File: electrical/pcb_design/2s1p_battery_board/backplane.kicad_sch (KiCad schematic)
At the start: 21 parts, among them J10 TE_Connectivity_7-5530843-7, J11 TE_Connectivity_7-5530843-7, J12 TE_Connectivity_7-5530843-7, J13 TE_Connectivity_7-5530843-7, J14 TE_Connectivity_7-5530843-7, J15 TE_Connectivity_7-5530843-7, J16 TE_Connectivity_7-5530843-7, J9 TE_Connectivity_7-5530843-7, U3 TCAN330

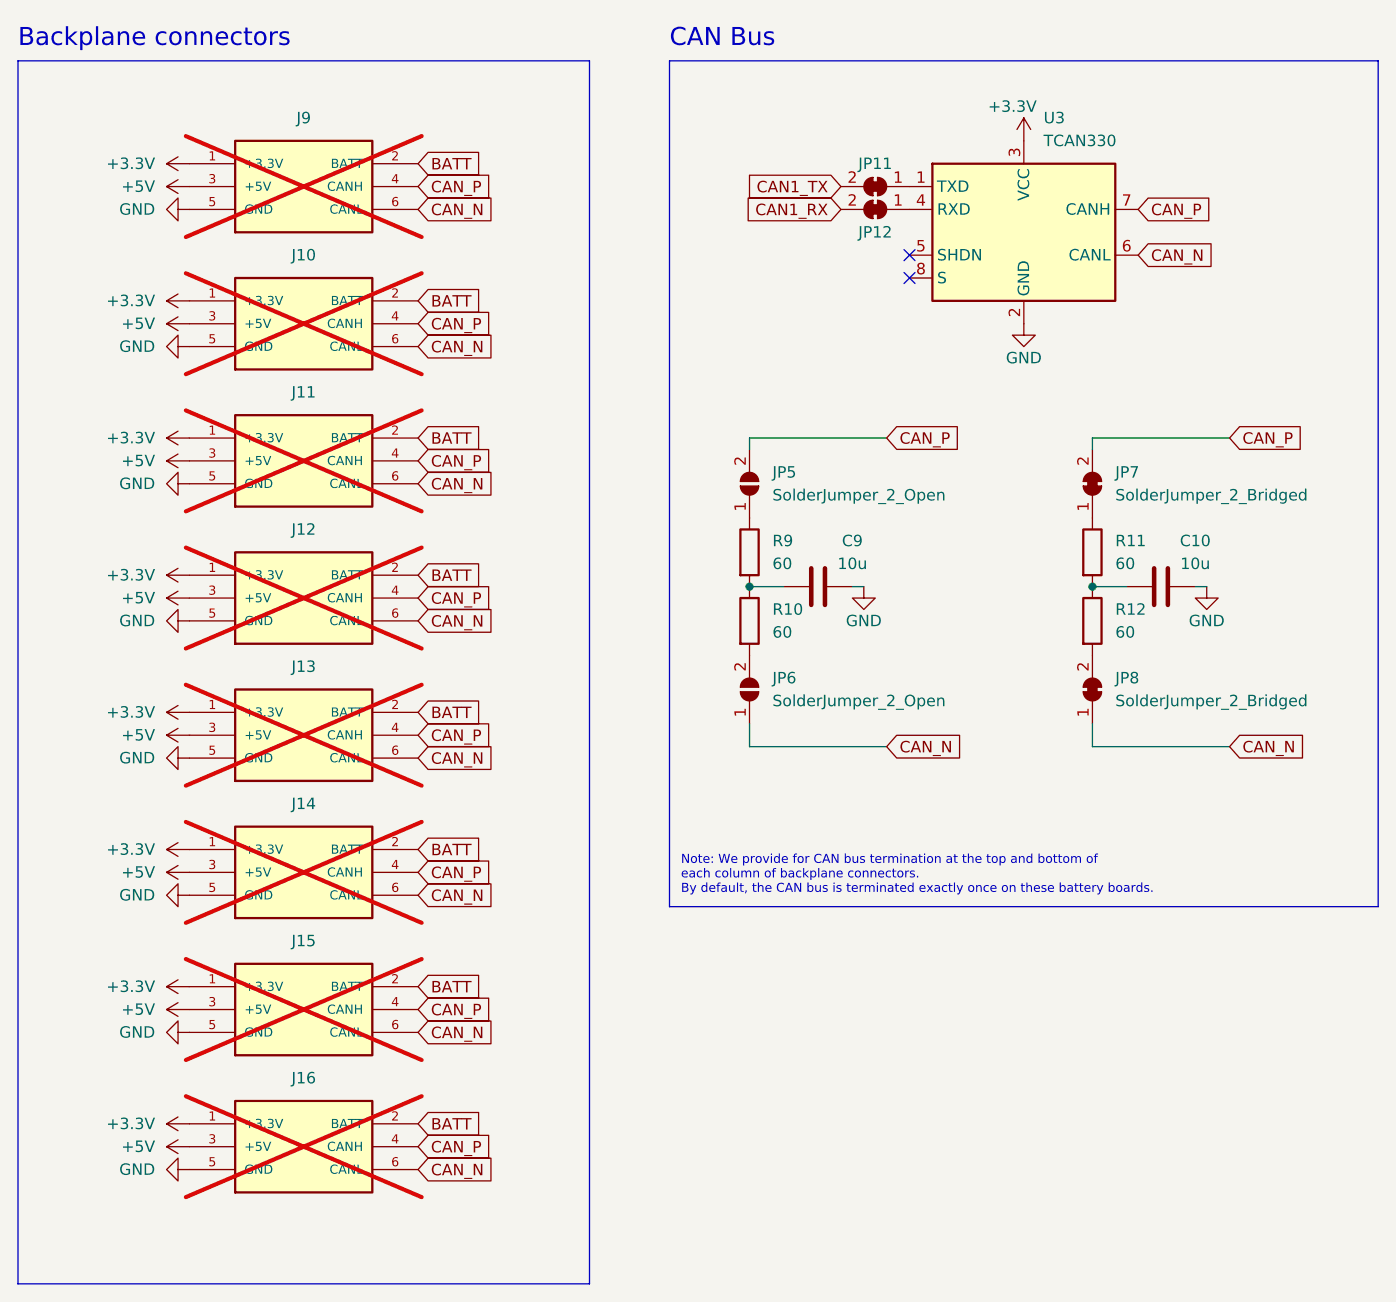
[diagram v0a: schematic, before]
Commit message: Checkpointing work rearranging backplane pin-out
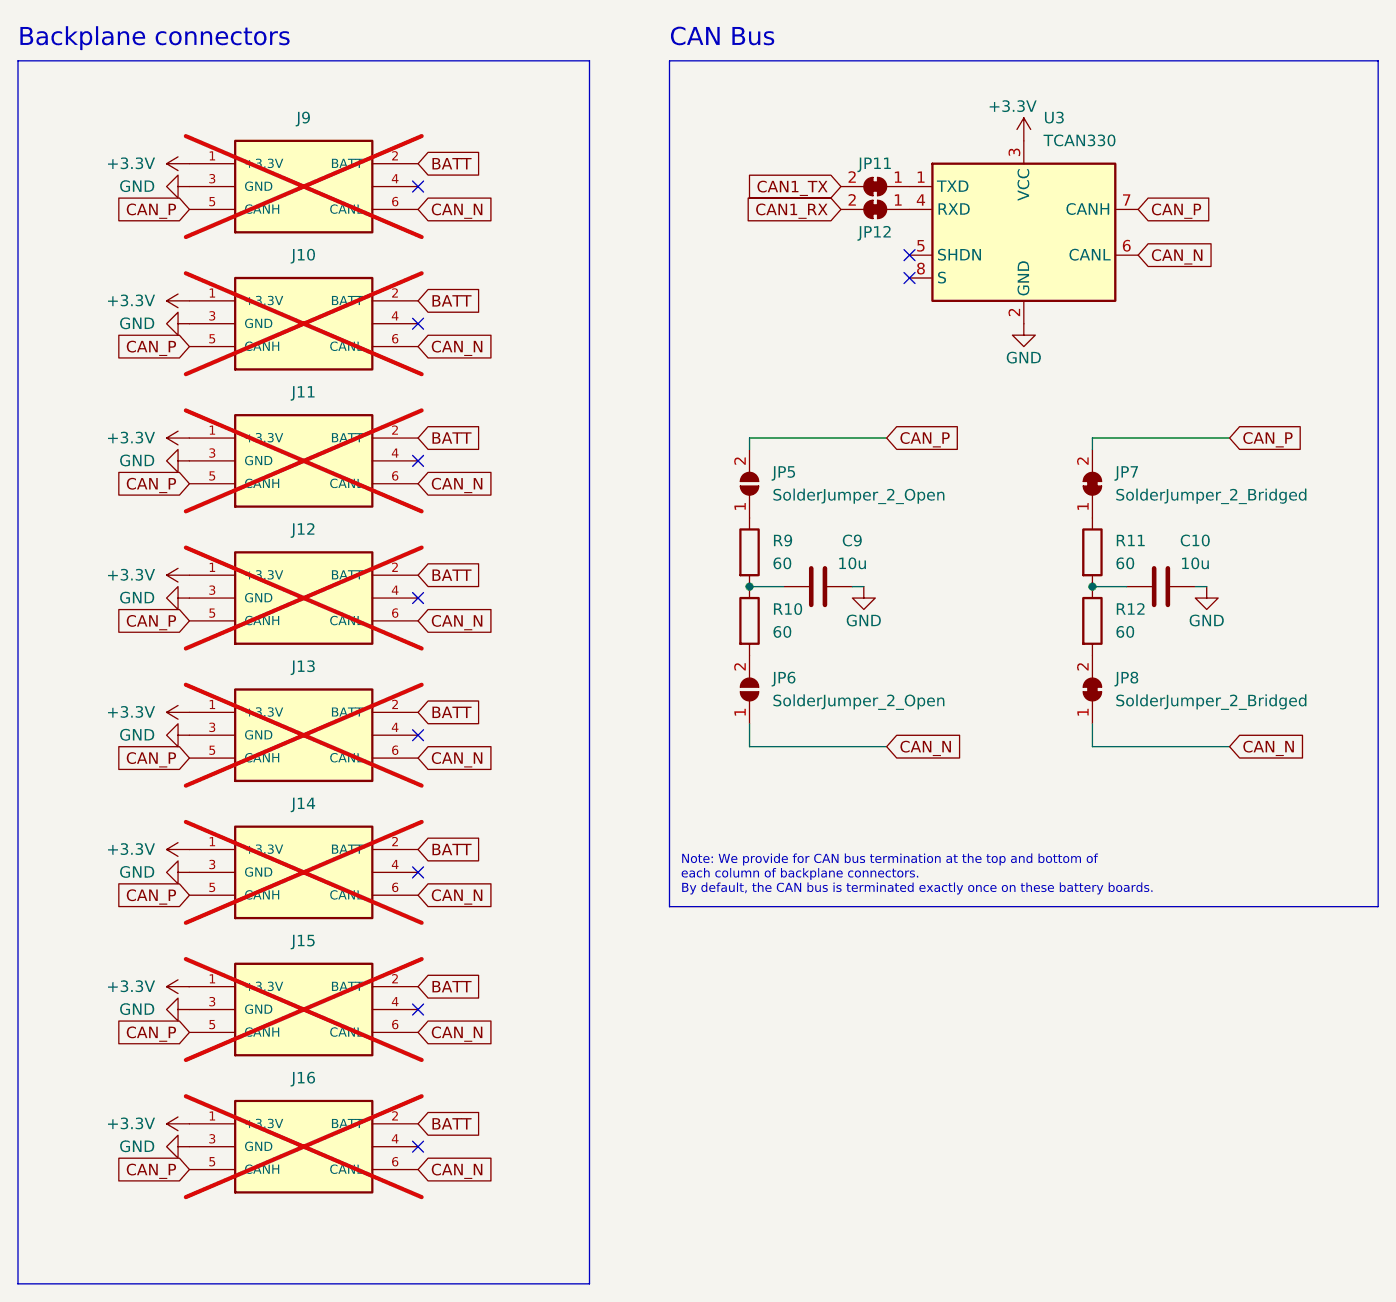
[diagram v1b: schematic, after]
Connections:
- net +5V is gone; now on net GND: J10.3 (GND), J11.3 (GND), J12.3 (GND), J13.3 (GND), J14.3 (GND), J15.3 (GND), J16.3 (GND), J9.3 (GND)
- net CAN_P: now also J10.5 (CANH), J11.5 (CANH), J12.5 (CANH), J13.5 (CANH), J14.5 (CANH), J15.5 (CANH), J16.5 (CANH), J9.5 (CANH); no longer J10.4 (CANH), J11.4 (CANH), J12.4 (CANH), J13.4 (CANH), J14.4 (CANH), J15.4 (CANH), J16.4 (CANH), J9.4 (CANH)
- net GND: no longer J10.5 (GND), J11.5 (GND), J12.5 (GND), J13.5 (GND), J14.5 (GND), J15.5 (GND), J16.5 (GND), J9.5 (GND)
- no-connect marks 2 -> 10
